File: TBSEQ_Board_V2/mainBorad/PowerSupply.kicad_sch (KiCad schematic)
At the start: 27 parts

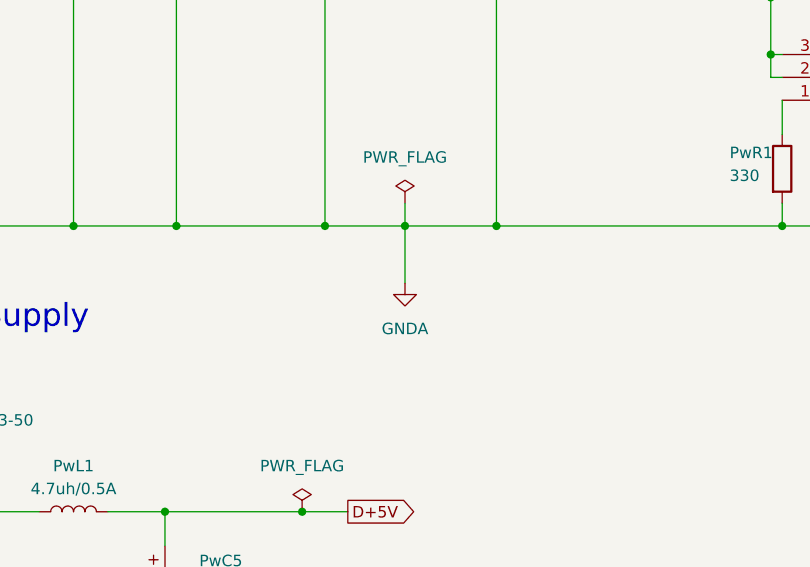
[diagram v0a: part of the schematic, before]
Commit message: mainBoard
AnInterface
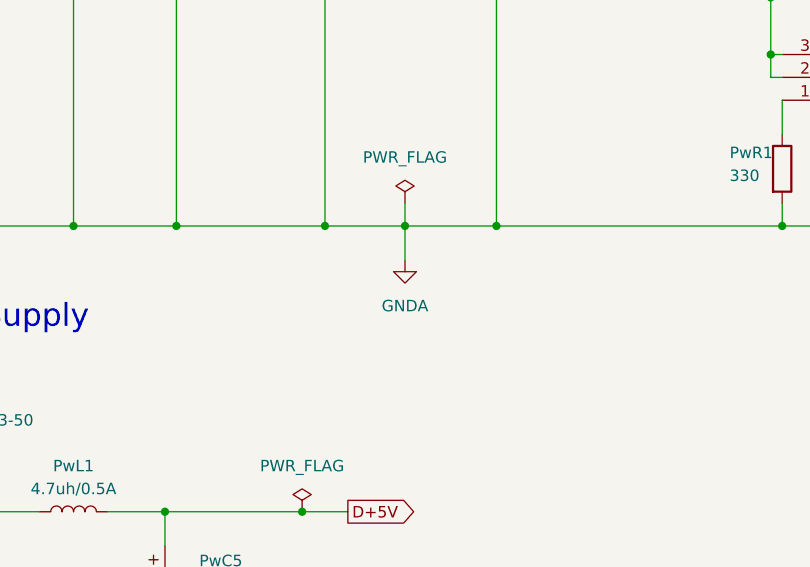
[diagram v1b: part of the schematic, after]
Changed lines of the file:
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@@
+	(wire
+		(pts
+			(xy 194.31 88.9) (xy 194.31 85.09)
+		)
+		(stroke
+			(width 0)
+			(type default)
+		)
+	)
 	(wire
 		(pts
@@
 		(pts
 			(xy 50.8 77.47) (xy 57.15 77.47)
-		)
-		(stroke
-			(width 0)
-			(type default)
-		)
-	)
-	(wire
-		(pts
-			(xy 194.31 91.44) (xy 194.31 85.09)
 		)
 		(stroke
@@
 	)
 	(symbol
+		(lib_id "power:GNDA")
+		(at 194.31 88.9 0)
+		(unit 1)
+		(exclude_from_sim no)
+		(in_bom yes)
+		(on_board yes)
+		(dnp no)
+		(fields_autoplaced yes)
+		(property "Reference" "#PWR018"
+			(at 194.31 95.25 0)
+			(effects
+				(font
+					(size 1.27 1.27)
+				)
+				(hide yes)
+			)
+		)
+		(property "Value" "GNDA"
+			(at 194.31 93.98 0)
+			(effects
+				(font
+					(size 1.27 1.27)
+				)
+			)
+		)
+		(property "Footprint" ""
+			(at 194.31 88.9 0)
+			(effects
+				(font
+					(size 1.27 1.27)
+				)
+				(hide yes)
+			)
+		)
+		(property "Datasheet" ""
+			(at 194.31 88.9 0)
+			(effects
+				(font
+					(size 1.27 1.27)
+				)
+				(hide yes)
+			)
+		)
+		(property "Description" "Power symbol creates a global label with name \"GNDA\" , analog ground"
+			(at 194.31 88.9 0)
+			(effects
+				(font
+					(size 1.27 1.27)
+				)
+				(hide yes)
+			)
+		)
+		(pin "1"
+		)
+		(instances
+			(project "mainBorad"
+				(path "/74b57c73-2ea6-4d1a-baa5-ad46186fbb51/d9cb4d85-ede2-449b-9b10-29aa5c34151e"
+					(reference "#PWR018")
+					(unit 1)
+				)
+			)
+		)
+	)
+	(symbol
 		(lib_id "Device:R")
 		(at 236.22 78.74 0)
@@
 					(unit 1)
 				)
-			)
-		)
-	)
-	(symbol
-		(lib_id "power:GNDA")
-		(at 194.31 91.44 0)
-		(unit 1)
-		(exclude_from_sim no)
-		(in_bom yes)
-		(on_board yes)
-		(dnp no)
-		(fields_autoplaced yes)
-		(property "Reference" "#PWR018"
-			(at 194.31 97.79 0)
-			(effects
-				(font
-					(size 1.27 1.27)
-				)
-				(hide yes)
-			)
-		)
-		(property "Value" "GNDA"
-			(at 194.31 96.52 0)
-			(effects
-				(font
-					(size 1.27 1.27)
-				)
-			)
-		)
-		(property "Footprint" ""
-			(at 194.31 91.44 0)
-			(effects
-				(font
-					(size 1.27 1.27)
-				)
-				(hide yes)
-			)
-		)
-		(property "Datasheet" ""
-			(at 194.31 91.44 0)
-			(effects
-				(font
-					(size 1.27 1.27)
-				)
-				(hide yes)
-			)
-		)
-		(property "Description" "Power symbol creates a global label with name \"GNDA\" , analog ground"
-			(at 194.31 91.44 0)
-			(effects
-				(font
-					(size 1.27 1.27)
-				)
-				(hide yes)
-			)
-		)
-		(pin "1"
-		)
-		(instances
-			(project "mainBorad"
-				(path "/74b57c73-2ea6-4d1a-baa5-ad46186fbb51/d9cb4d85-ede2-449b-9b10-29aa5c34151e"
-					(reference "#PWR018")
-					(unit 1)
-				)
